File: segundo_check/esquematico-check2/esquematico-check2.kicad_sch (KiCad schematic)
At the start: 21 parts, among them J1 Conn_01x02, J2 Conn_01x02, Q1 BC547, Q2 BC547, Q3 BC547, Q4 BC557, Q5 BC557, Q6 MJE2955T, Q7 BC547, Q8 BC547, Q9 BC547, U1 TL431D

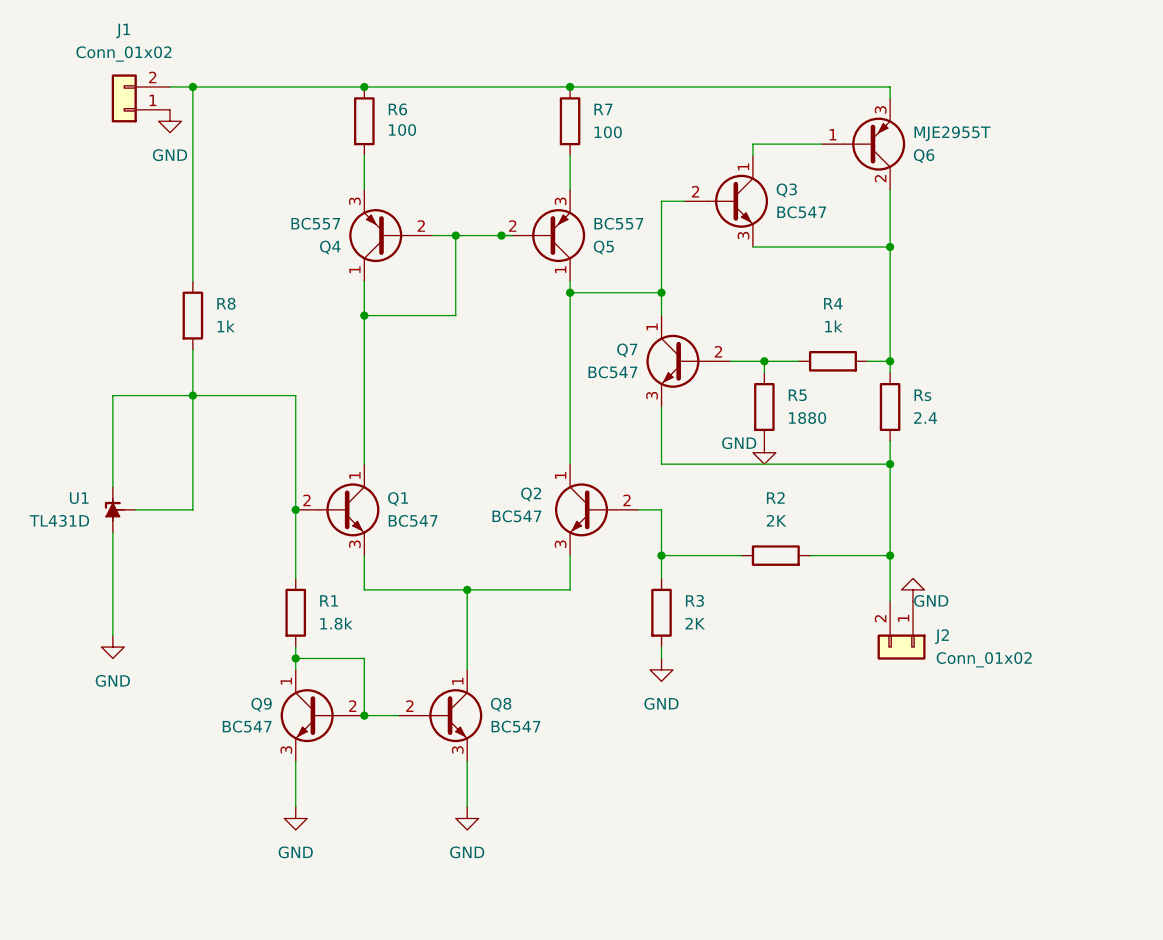
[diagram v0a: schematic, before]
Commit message: Avances PCB
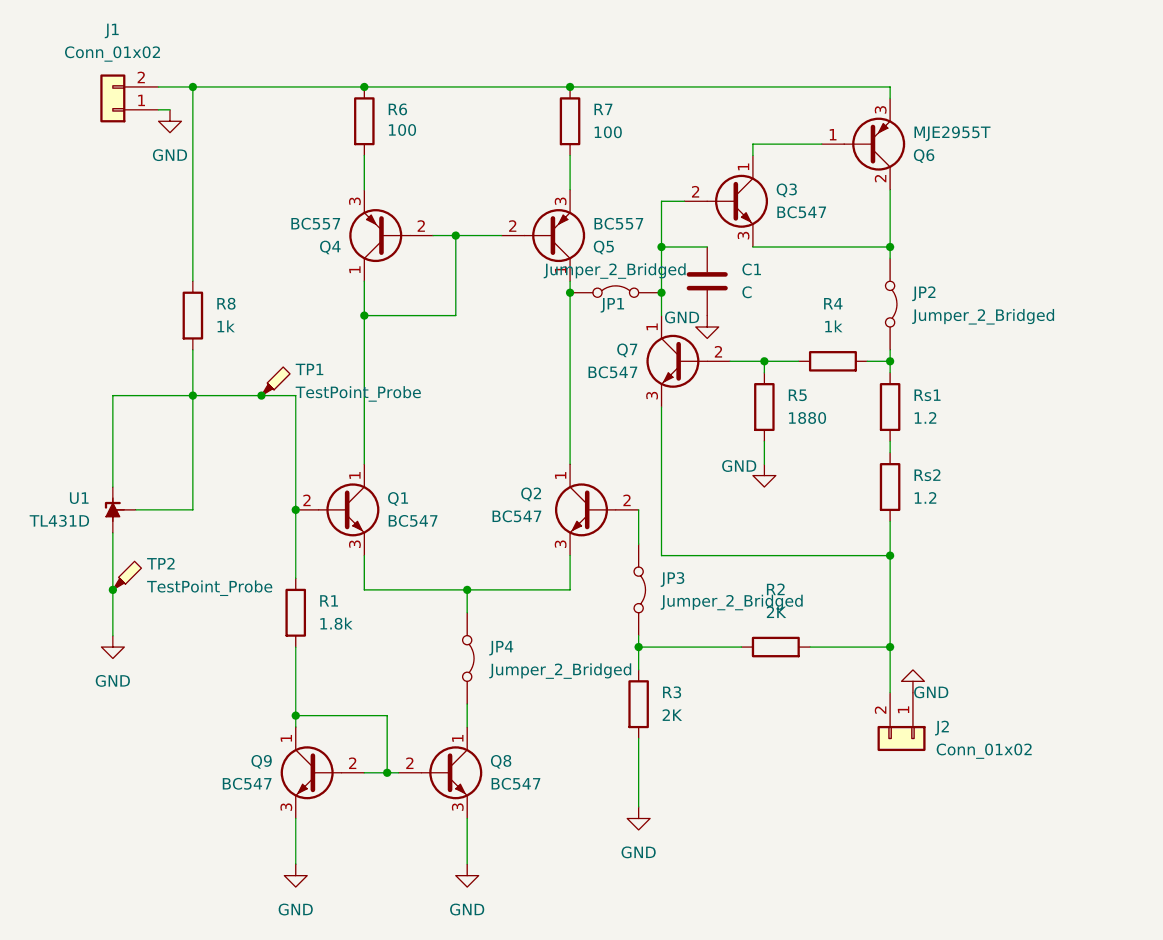
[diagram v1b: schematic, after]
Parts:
- added C1: C, Capacitor_THT:C_Rect_L9.0mm_W4.0mm_P7.50mm_MKT, symbol Device:C
- added JP1, JP2, JP3, JP4: Jumper_2_Bridged, TestPoint:TestPoint_2Pads_Pitch2.54mm_Drill0.8mm, symbol Jumper:Jumper_2_Bridged
- added Rs2: 1.2, Resistor_THT:R_Axial_Power_L25.0mm_W9.0mm_P30.48mm, symbol Device:R
- added TP1, TP2: TestPoint_Probe, TestPoint:TestPoint_Keystone_5000-5004_Miniature, symbol Connector:TestPoint_Probe
- J1, J2: footprint (none) -> Connector_Samtec_HPM_THT:Samtec_HPM-02-01-x-S_Straight_1x02_Pitch5.08mm
- R1, R2, R3, R4, R5, R6, R7, R8: footprint (none) -> Resistor_THT:R_Axial_DIN0207_L6.3mm_D2.5mm_P10.16mm_Horizontal
- Rs1: renamed from Rs; value 2.4 -> 1.2; footprint (none) -> Resistor_THT:R_Axial_Power_L25.0mm_W9.0mm_P30.48mm
- U1: footprint Package_SO:SOIC-8_3.9x4.9mm_P1.27mm -> Package_TO_SOT_THT:TO-92_Inline_Wide
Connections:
- net GND: now also C1.2, TP2.1
- net at R4.2, Rs1.1: now also JP2.2 (B); no longer Q3.3 (E), Q6.2 (C)
- net at Q2.1 (C), Q5.1 (C): now also JP1.1 (A); no longer Q3.2 (B), Q7.1 (C)
- net at R2.1, R3.1: now also JP3.2 (B); no longer Q2.2 (B)
- net at Q1.3 (E), Q2.3 (E): now also JP4.1 (A); no longer Q8.1 (C)
- net at J2.2 (Pin_2), Q7.3 (E), R2.2: now also Rs2.2; no longer Rs1.2
- net at Q1.2 (B), R1.1, R8.2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: now also TP1.1
- new net: Rs1.2, Rs2.1
- new net: C1.1, JP1.2 (B), Q3.2 (B), Q7.1 (C)
- new net: JP3.1 (A), Q2.2 (B)
- new net: JP4.2 (B), Q8.1 (C)
- new net: JP2.1 (A), Q3.3 (E), Q6.2 (C)
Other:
- moved on the sheet: J1, J2, Q8, Q9, R2, R3

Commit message: Placa reglin terminada?
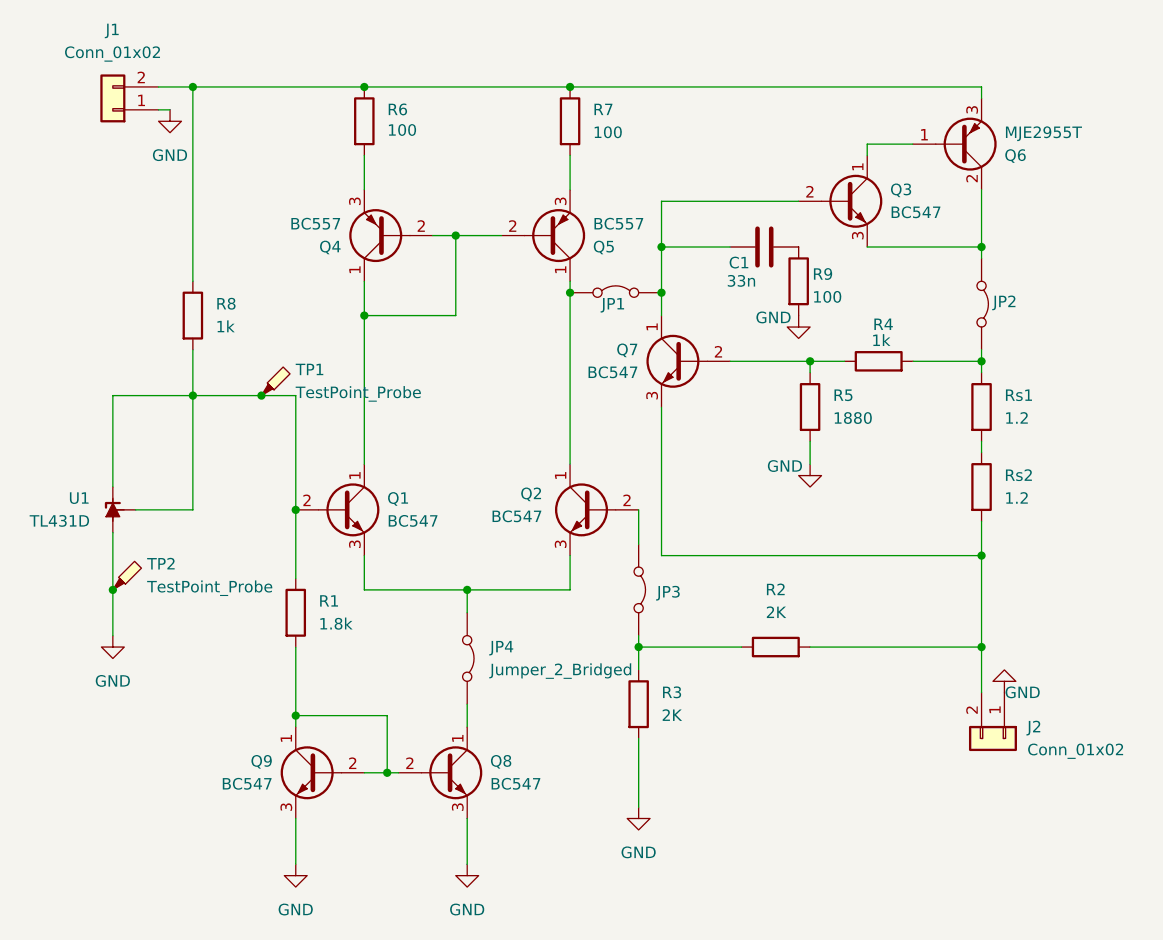
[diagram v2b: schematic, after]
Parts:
- added R9: 100, Resistor_THT:R_Axial_DIN0204_L3.6mm_D1.6mm_P5.08mm_Horizontal, symbol Device:R
- C1: value C -> 33n; footprint Capacitor_THT:C_Rect_L9.0mm_W4.0mm_P7.50mm_MKT -> Capacitor_THT:C_Disc_D4.3mm_W1.9mm_P5.00mm
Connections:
- net GND: now also R9.2; no longer C1.2
- new net: C1.2, R9.1
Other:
- moved on the sheet: J2, JP2, Q3, Q6, R4, R5, Rs1, Rs2
